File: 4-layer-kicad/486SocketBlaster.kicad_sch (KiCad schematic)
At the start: 16 parts, among them U1 TPS563200

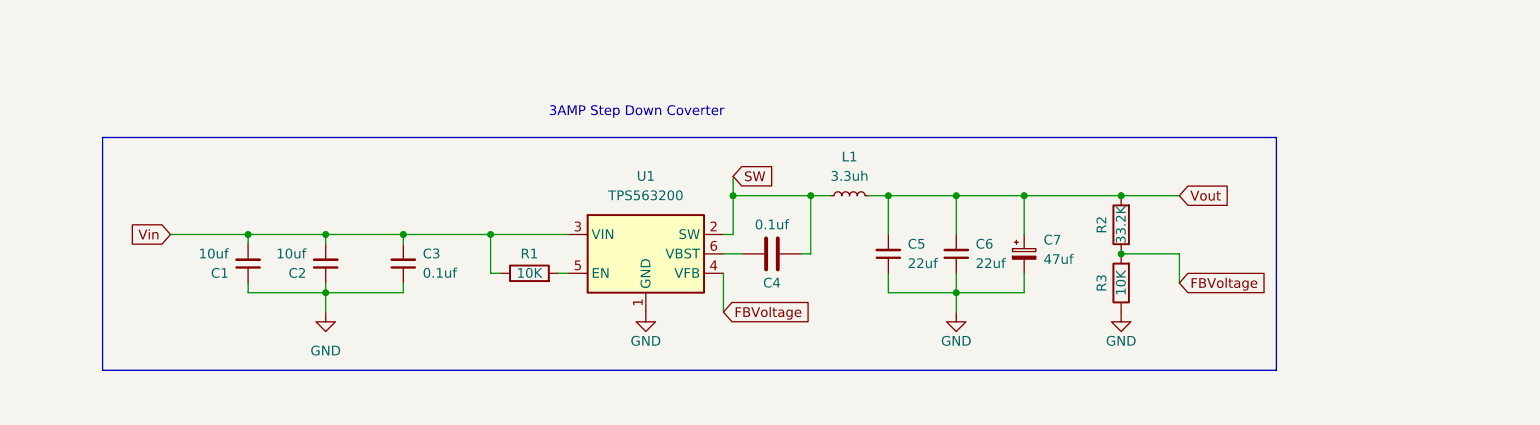
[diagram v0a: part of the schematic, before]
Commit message: update
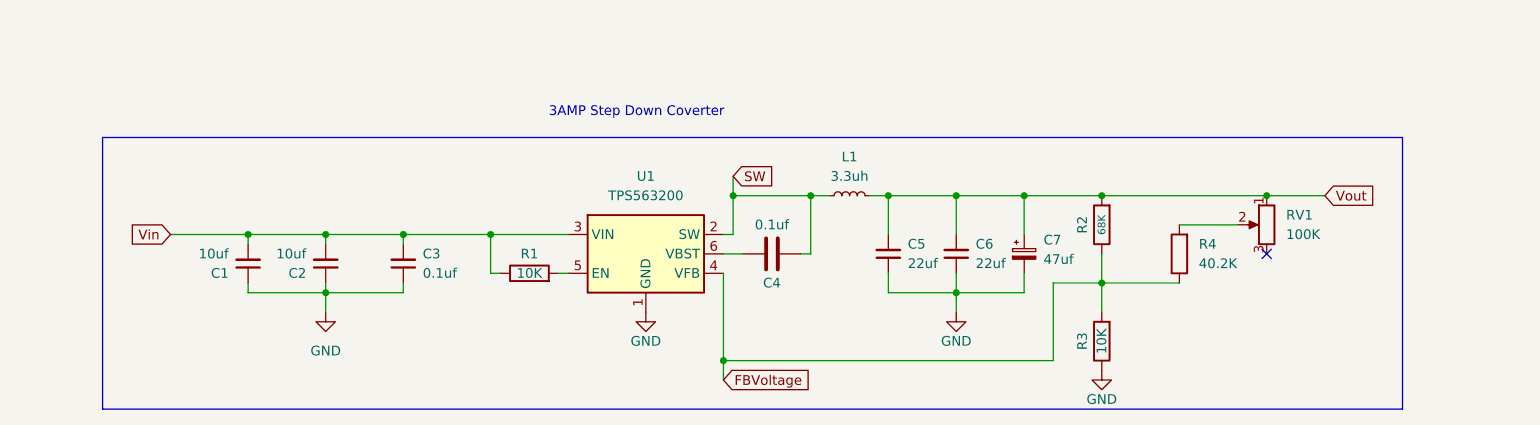
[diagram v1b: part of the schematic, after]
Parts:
- added R4: 40.2K, 486SocketBlaster:R_0603_1608Metric, symbol Device:R
- added RV1: 100K, 486SocketBlaster:tinySMDpot, symbol Device:R_Potentiometer
- R2: value 33.2K -> 68K; JLCPCB C4216 -> (none); JLCPCB for set (none) -> C4216; Set valie (none) -> 33.2K; adj value (none) -> 68K
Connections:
- net FBVoltage: now also R4.1
- net Vout: now also RV1.1
- new net: R4.2, RV1.2
- no-connect marks 0 -> 1
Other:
- moved on the sheet: R2, R3

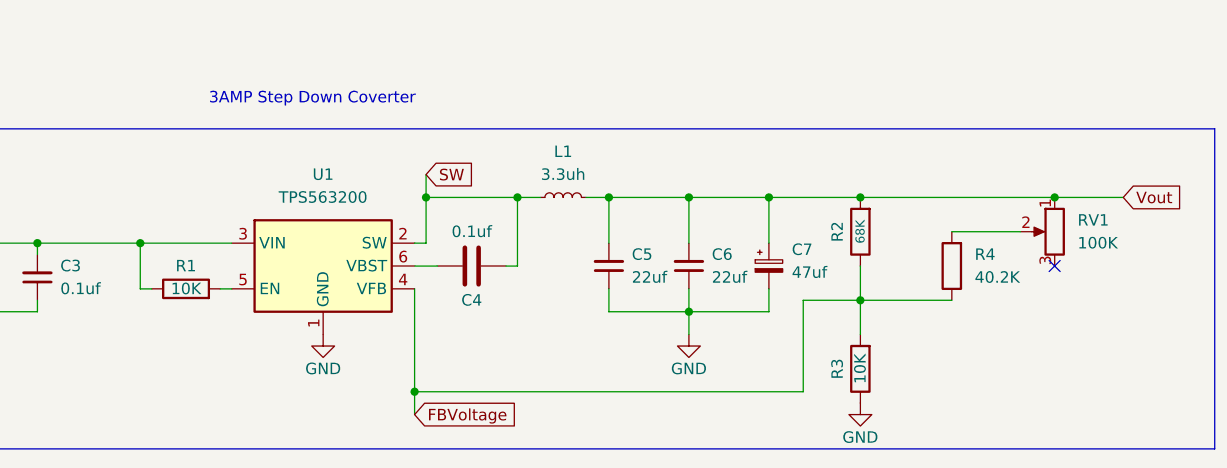
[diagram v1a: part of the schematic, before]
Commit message: update
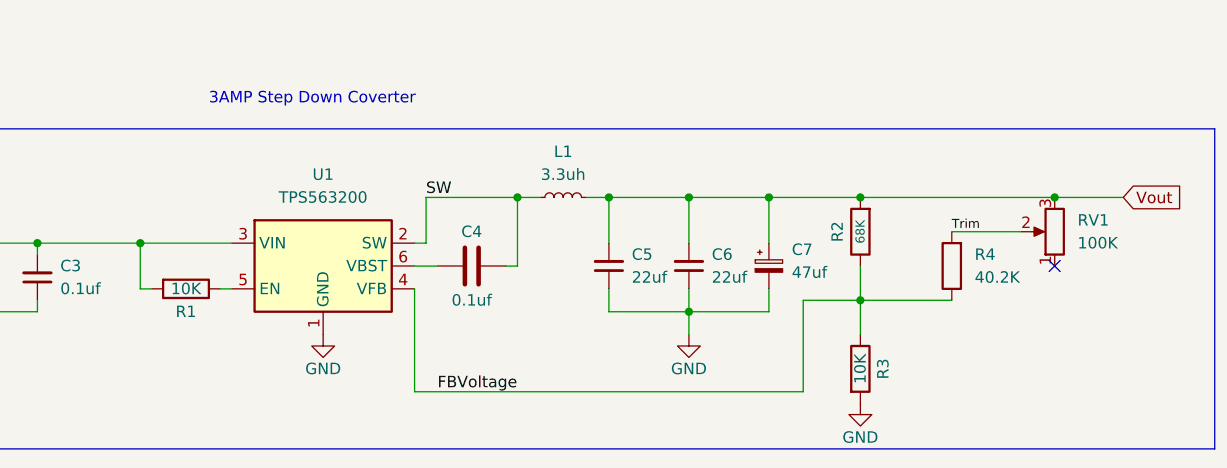
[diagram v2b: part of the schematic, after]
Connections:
- net FBVoltage: now also R3.1; no longer R3.2
- net GND: now also R3.2; no longer R3.1
- net SW: now also C4.2; no longer C4.1
- net Vin: now also R1.2; no longer R1.1
- net Vout: now also RV1.3; no longer RV1.1
- net at U1.6 (VBST): now also C4.1; no longer C4.2
- net at U1.5 (EN): now also R1.1; no longer R1.2
- net Trim: now reaches R4.2, RV1.2
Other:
- moved on the sheet: C4, R1, R3, RV1
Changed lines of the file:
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@@
   (junction (at 488.95 63.5) (diameter 0) (color 0 0 0 0)
   )
+  (junction (at 233.68 153.67) (diameter 0) (color 0 0 0 0)
+  )
   (junction (at 285.75 63.5) (diameter 0) (color 0 0 0 0)
   )
@@
   (junction (at 318.77 63.5) (diameter 0) (color 0 0 0 0)
   )
-  (junction (at 162.56 175.26) (diameter 0) (color 0 0 0 0)
-  )
   (junction (at 483.87 63.5) (diameter 0) (color 0 0 0 0)
   )
@@
   (junction (at 236.22 38.1) (diameter 0) (color 0 0 0 0)
   )
-  (junction (at 163.83 153.67) (diameter 0) (color 0 0 0 0)
-  )
   (junction (at 120.65 158.75) (diameter 0) (color 0 0 0 0)
   )
@@
   )
   (junction (at 336.55 88.9) (diameter 0) (color 0 0 0 0)
-  )
-  (junction (at 233.68 153.67) (diameter 0) (color 0 0 0 0)
   )
   (junction (at 448.31 88.9) (diameter 0) (color 0 0 0 0)
@@
     (stroke (width 0) (type default) (color 0 0 0 0))
   )
-  (wire (pts (xy 162.56 175.26) (xy 162.56 177.8))
-    (stroke (width 0) (type default) (color 0 0 0 0))
-  )
   (wire (pts (xy 499.11 63.5) (xy 514.35 63.5))
     (stroke (width 0) (type default) (color 0 0 0 0))
@@
     (stroke (width 0) (type default) (color 0 0 0 0))
   )
-  (wire (pts (xy 163.83 151.13) (xy 163.83 153.67))
-    (stroke (width 0) (type default) (color 0 0 0 0))
-  )
   (wire (pts (xy 229.87 57.15) (xy 229.87 53.34))
     (stroke (width 0) (type default) (color 0 0 0 0))
@@
     (stroke (width 0) (type default) (color 0 0 0 0))
   )
+  (wire (pts (xy 233.68 153.67) (xy 241.3 153.67))
+    (stroke (width 0) (type default) (color 0 0 0 0))
+  )
   (wire (pts (xy 146.05 88.9) (xy 151.13 88.9))
     (stroke (width 0) (type default) (color 0 0 0 0))
@@
   )
   (wire (pts (xy 335.28 57.15) (xy 336.55 57.15))
-    (stroke (width 0) (type default) (color 0 0 0 0))
-  )
-  (wire (pts (xy 233.68 153.67) (xy 241.3 153.67))
     (stroke (width 0) (type default) (color 0 0 0 0))
   )
@@
   (text "3AMP Step Down Coverter" (at 139.7 143.51 0)
     (effects (font (size 1.27 1.27)) (justify left bottom))
+  )
+  (label "FBVoltage" (at 165.1 175.26 0)
+    (effects (font (size 1.27 1.27)) (justify left bottom))
+  )
+  (label "SW" (at 163.83 153.67 0)
+    (effects (font (size 1.27 1.27)) (justify left bottom))
+  )
+  (label "Trim" (at 222.25 157.48 0)
+    (effects (font (size 1 1)) (justify left bottom))
   )
   (global_label "Vout" (shape input) (at 241.3 153.67 0) (fields_autoplaced)
@@
     )
   )
-  (global_label "SW" (shape input) (at 163.83 151.13 0) (fields_autoplaced)
-    (effects (font (size 1.27 1.27)) (justify left))
-    (property "Intersheet References" "${INTERSHEET_REFS}" (id 0) (at 168.9041 151.0506 0)
-      (effects (font (size 1.27 1.27)) (justify left) hide)
-    )
-  )
   (global_label "Vin" (shape input) (at 90.17 158.75 180) (fields_autoplaced)
     (effects (font (size 1.27 1.27)) (justify right))
@@
     (effects (font (size 1.27 1.27)) (justify left))
     (property "Intersheet References" "${INTERSHEET_REFS}" (id 0) (at 303.6166 30.4006 0)
-      (effects (font (size 1.27 1.27)) (justify left) hide)
-    )
-  )
-  (global_label "FBVoltage" (shape input) (at 162.56 177.8 0) (fields_autoplaced)
-    (effects (font (size 1.27 1.27)) (justify left))
-    (property "Intersheet References" "${INTERSHEET_REFS}" (id 0) (at 174.3469 177.7206 0)
       (effects (font (size 1.27 1.27)) (justify left) hide)
     )
@@
     (pin "3")
   )
-  (symbol (lib_id "Device:C") (at 168.91 161.29 270) (unit 1)
+  (symbol (lib_id "Device:C") (at 168.91 161.29 90) (unit 1)
     (in_bom yes) (on_board yes)
-    (property "Reference" "C4" (id 0) (at 168.91 165.1 90))
-    (property "Value" "0.1uf" (id 1) (at 168.91 157.48 90))
-    (property "Footprint" "486SocketBlaster:C_0603_1608Metric" (id 2) (at 165.1 162.2552 0)
+    (property "Reference" "C4" (id 0) (at 168.91 157.48 90))
+    (property "Value" "0.1uf" (id 1) (at 168.91 165.1 90))
+    (property "Footprint" "486SocketBlaster:C_0603_1608Metric" (id 2) (at 172.72 160.3248 0)
       (effects (font (size 1.27 1.27)) hide)
     )
@@
     (pin "2")
   )
-  (symbol (lib_id "Device:R") (at 137.16 163.83 90) (unit 1)
+  (symbol (lib_id "Device:R") (at 137.16 163.83 270) (unit 1)
     (in_bom yes) (on_board yes)
-    (property "Reference" "R1" (id 0) (at 137.16 161.29 90))
+    (property "Reference" "R1" (id 0) (at 137.16 166.37 90))
     (property "Value" "10K" (id 1) (at 137.16 163.83 90))
-    (property "Footprint" "486SocketBlaster:R_0603_1608Metric" (id 2) (at 137.16 165.608 90)
+    (property "Footprint" "486SocketBlaster:R_0603_1608Metric" (id 2) (at 137.16 162.052 90)
       (effects (font (size 1.27 1.27)) hide)
     )
@@
     (pin "2")
   )
-  (symbol (lib_id "Device:R_Potentiometer") (at 233.68 157.48 0) (mirror y) (unit 1)
+  (symbol (lib_id "Device:R_Potentiometer") (at 233.68 157.48 180) (unit 1)
     (in_bom yes) (on_board yes) (fields_autoplaced)
     (property "Reference" "RV1" (id 0) (at 236.22 156.2099 0)
@@
     (pin "1")
   )
-  (symbol (lib_id "Device:R") (at 212.09 172.72 180) (unit 1)
+  (symbol (lib_id "Device:R") (at 212.09 172.72 0) (unit 1)
     (in_bom yes) (on_board yes)
-    (property "Reference" "R3" (id 0) (at 209.55 172.72 90))
+    (property "Reference" "R3" (id 0) (at 214.63 172.72 90))
     (property "Value" "10K" (id 1) (at 212.09 172.72 90))
-    (property "Footprint" "486SocketBlaster:R_0603_1608Metric" (id 2) (at 213.868 172.72 90)
-      (effects (font (size 1.27 1.27)) hide)
-    )
+    (property "Footprint" "486SocketBlaster:R_0603_1608Metric" (id 2) (at 210.312 172.72 90)
+      (effects (font (size 1.27 1.27)) hide)
+    )
